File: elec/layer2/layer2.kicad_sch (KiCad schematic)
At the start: 1 part

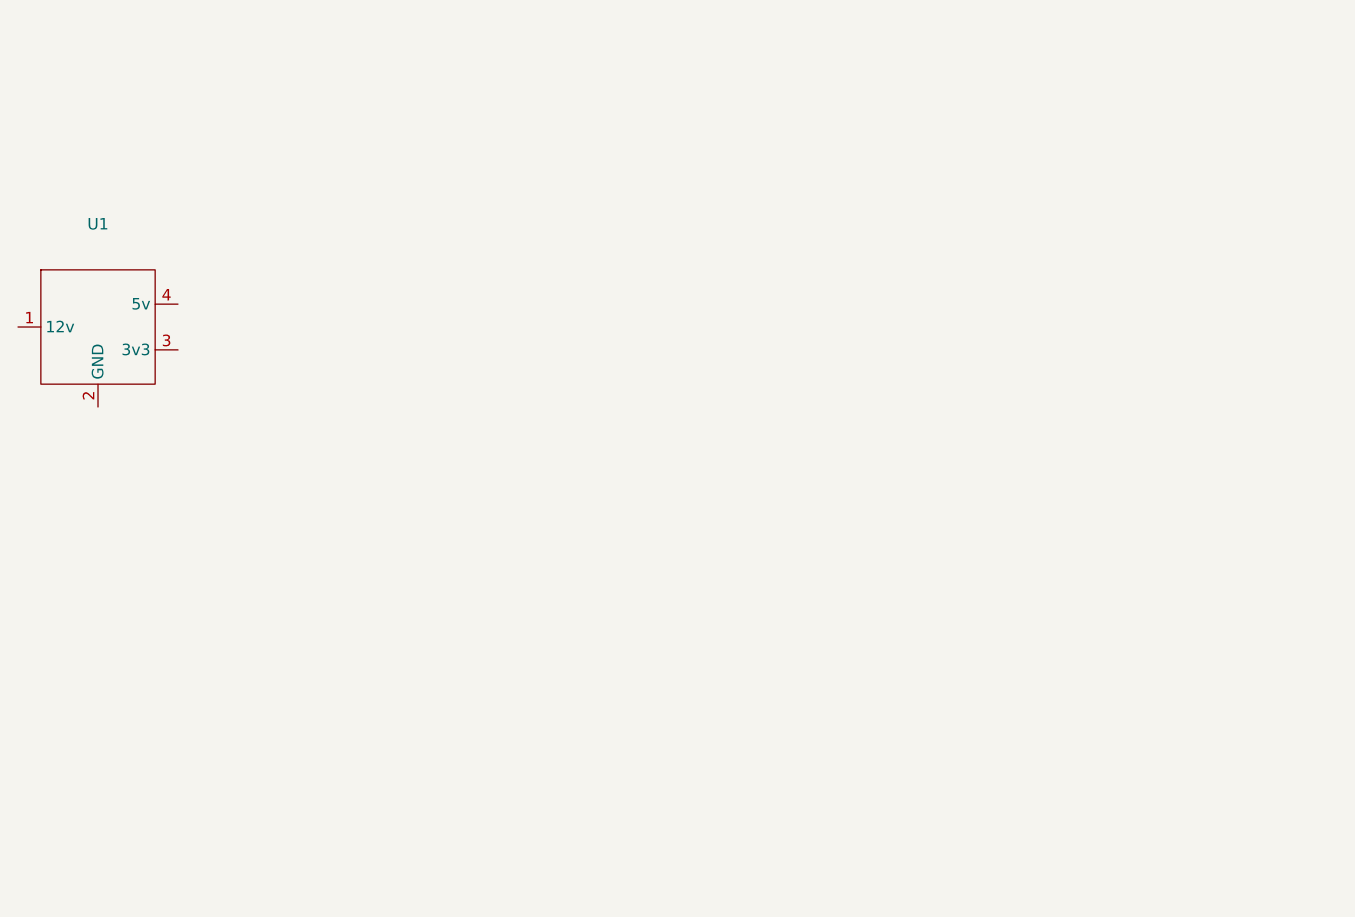
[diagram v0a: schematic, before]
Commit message: feat: did something
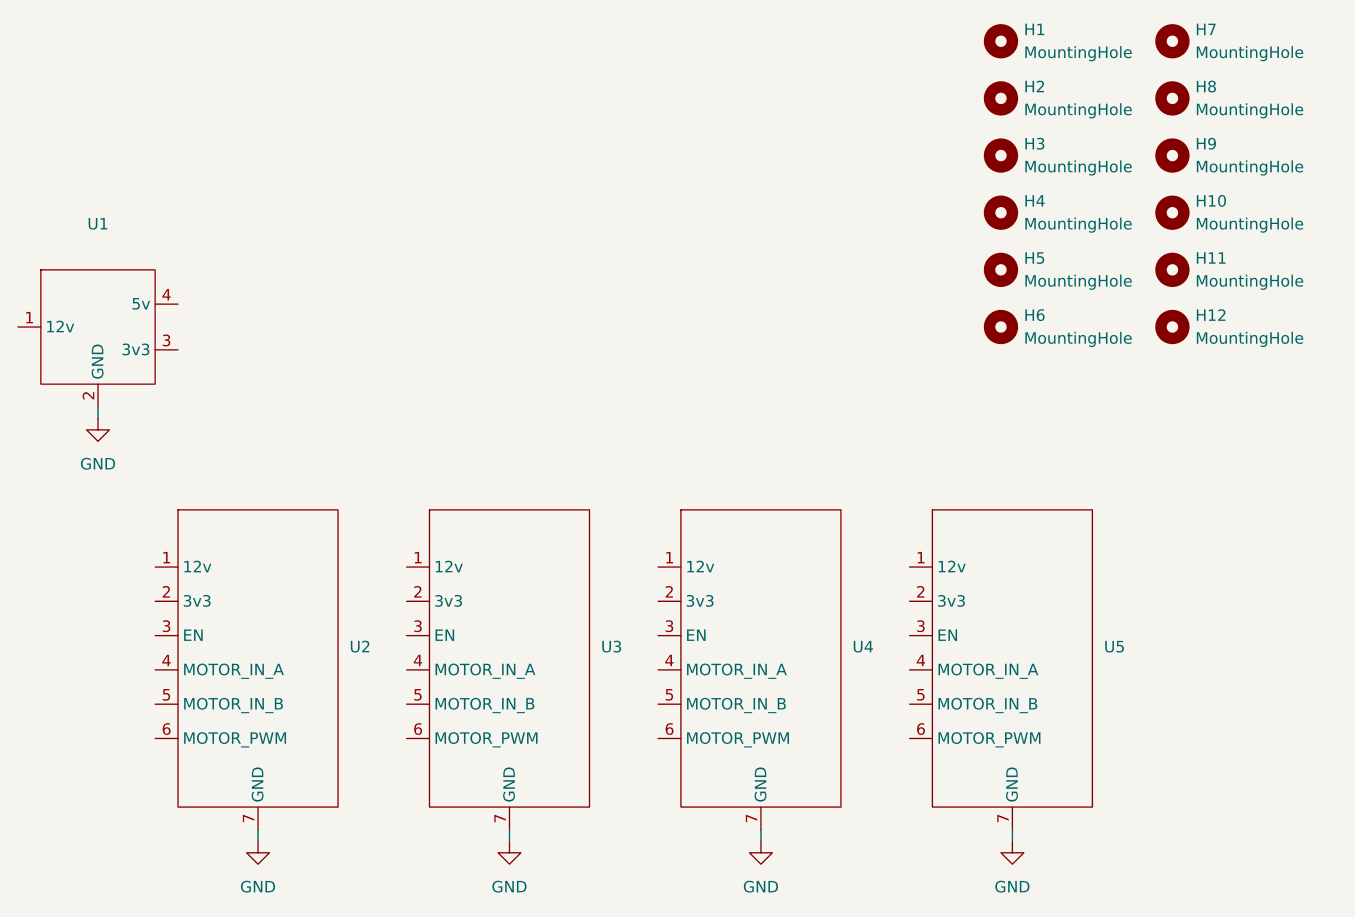
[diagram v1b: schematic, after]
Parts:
- added H1, H10, H11, H12, H2, H3, H4, H5, H6, H7, H8, H9: MountingHole, MountingHole:MountingHole_3.2mm_M3_DIN965_Pad, symbol Mechanical:MountingHole
- added U2, U3, U4, U5: ~, layer2-pcb-footprints:motor-driver-module, symbol layer2-pcb-symbols:motor-driver-module
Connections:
- net GND: now reaches U1.2 (GND)
- net GND: now also U2.7 (GND), U3.7 (GND), U4.7 (GND), U5.7 (GND)
